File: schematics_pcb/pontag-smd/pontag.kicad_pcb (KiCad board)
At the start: 2 copper layers, 31 parts, among them J1 External 5V, J2 External 12V, J3 RS232 Port, J4 PS/2 Mouse, J5 ISP, J7 Extra, SW1 Reset, U1 LP2985-5.0, U3 ATmega8A-AU, U4 MAX232A, Y1 8.0Mhz

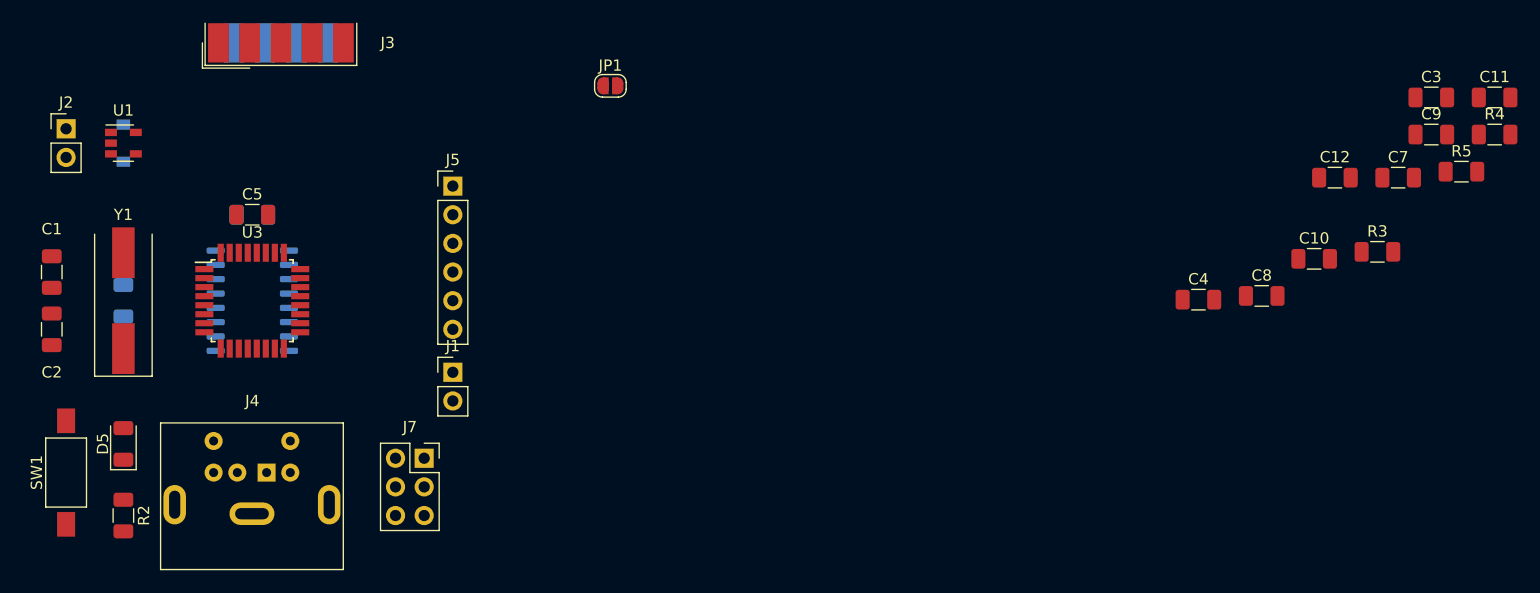
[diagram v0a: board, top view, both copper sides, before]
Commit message: Go on with board routing
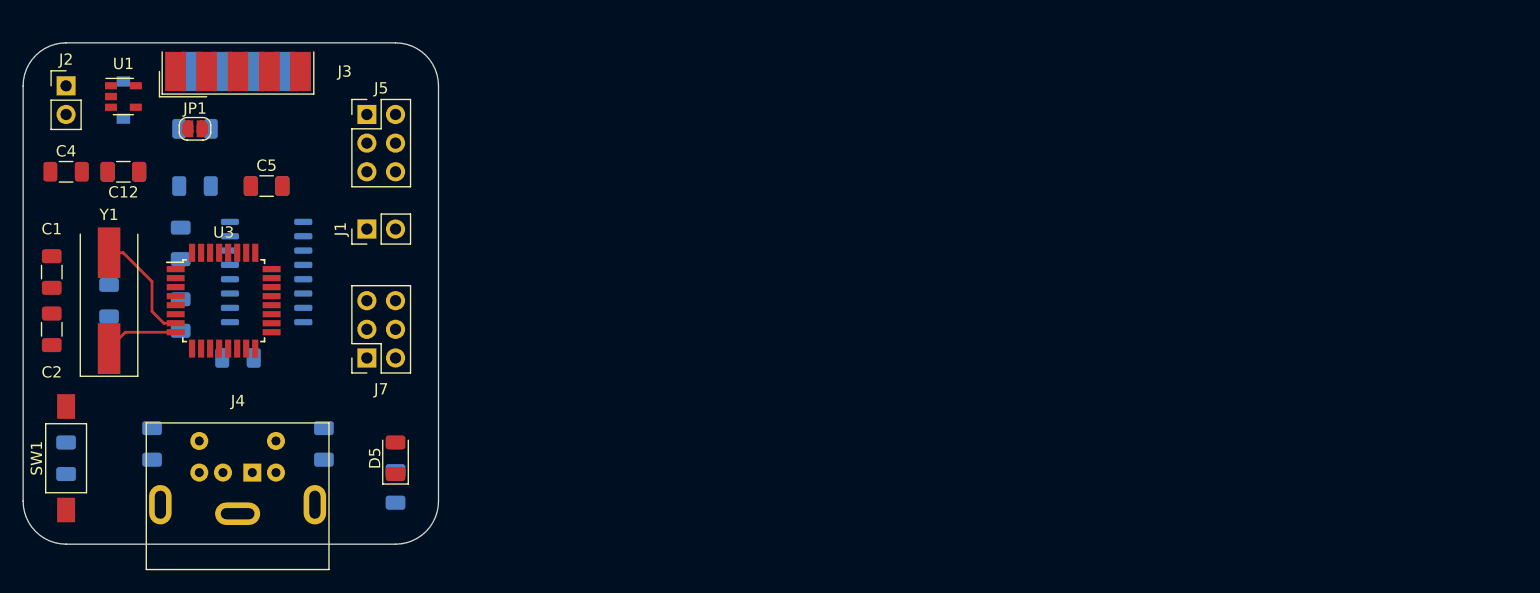
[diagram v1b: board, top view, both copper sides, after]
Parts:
- C10, C11, C3, C7, C8, C9, R2, R3, R4, R5: moved to B.Cu
- J5: value ISP -> AVR-ISP-6; footprint Connector_PinHeader_2.54mm:PinHeader_1x06_P2.54mm_Vertical -> Connector_PinHeader_2.54mm:PinHeader_2x03_P2.54mm_Vertical
- moved R5 126.3 mm to (67.3, 133.3), turned to 270 degrees
- moved C3 116.2 mm to (72.4, 108.0)
- moved C11 115.5 mm to (78.7, 109.2)
- moved C9 111.3 mm to (77.5, 114.3), turned to 90 degrees
- moved R3 110.0 mm to (74.9, 132.1), turned to 90 degrees
- moved C12 107.4 mm to (72.4, 108.0), turned to 180 degrees
- moved R4 107.4 mm to (90.2, 132.1), turned to 270 degrees
- moved C7 106.8 mm to (78.7, 104.1), turned to 180 degrees
- moved C4 101.0 mm to (67.3, 108.0)
- moved C8 95.9 mm to (77.5, 120.7), turned to 90 degrees
- moved C10 95.8 mm to (82.5, 124.5)
- moved JP1 37.0 mm to (78.7, 104.1)
- moved R2 24.3 mm to (96.5, 135.9)
- moved D5 24.2 mm to (96.5, 133.3)
- moved J1 14.8 mm to (94.0, 113.0), turned to 90 degrees
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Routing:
- net /XTAL1: track 0.00 -> 10.0 mm
- net /XTAL2: track 0.00 -> 6.51 mm
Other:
- board outline added: 36.8 x 44.5 mm

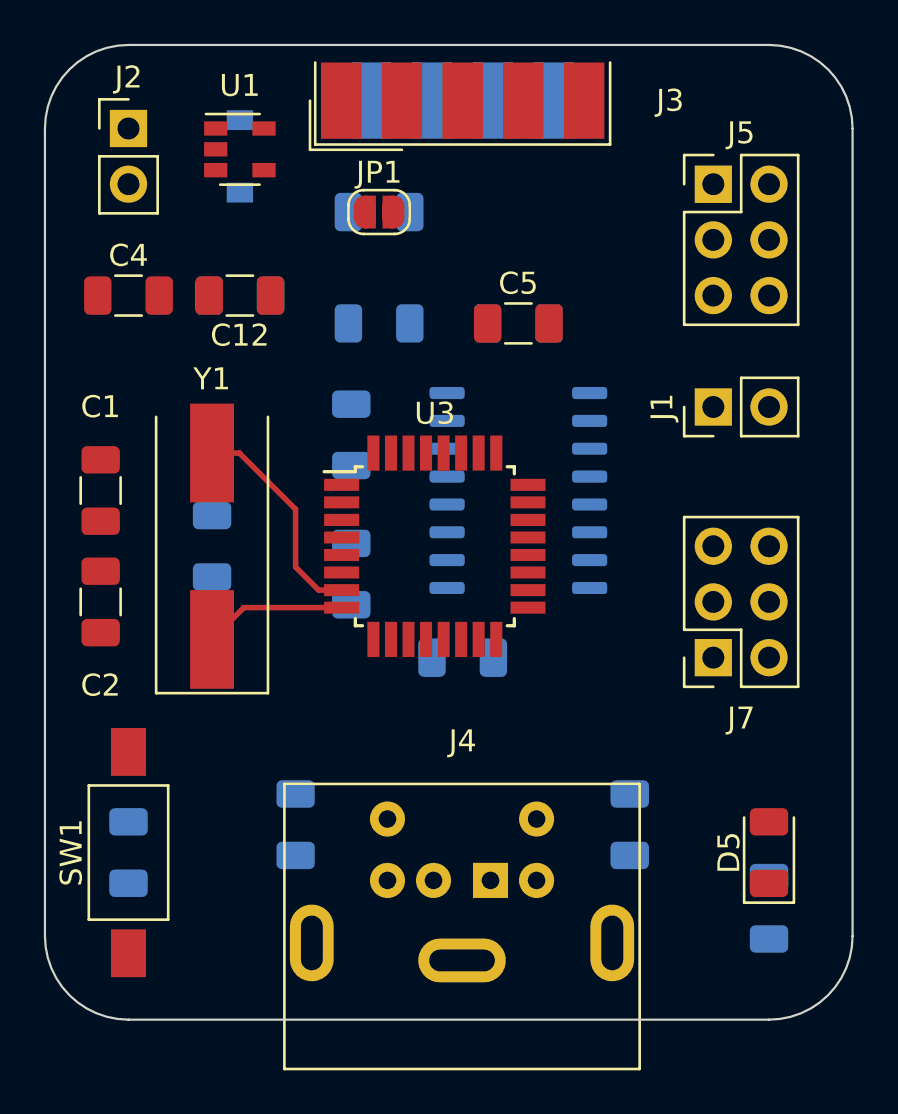
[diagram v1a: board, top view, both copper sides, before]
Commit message: Updates on SMD PCB
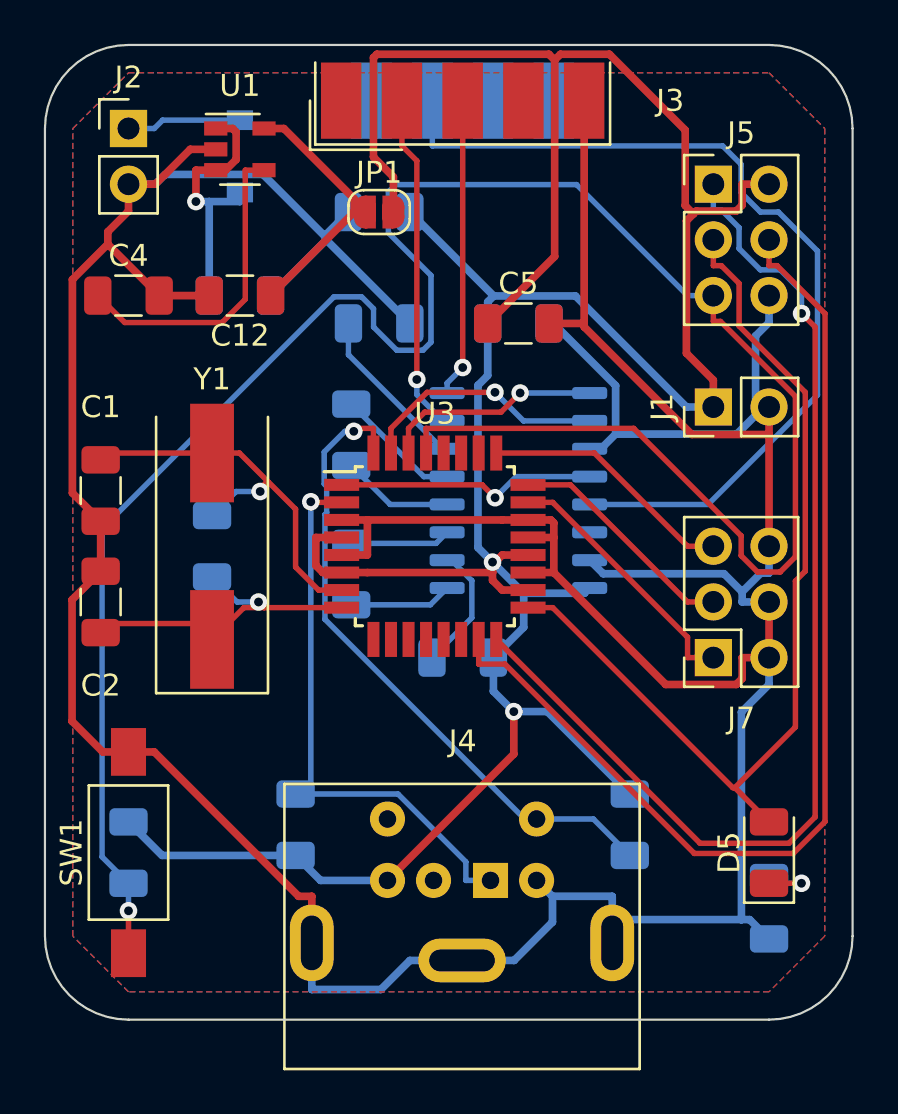
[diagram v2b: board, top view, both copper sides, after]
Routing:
- net GND: track 0.00 -> 210.0 mm
- net VCC: track 0.00 -> 141.2 mm, vias 0 -> 2
- net /RESET: track 0.00 -> 100.7 mm, vias 0 -> 1
- net /MISO: track 0.00 -> 50.4 mm, vias 0 -> 1
- net /MOSI: track 0.00 -> 48.9 mm
- net /SCK: track 0.00 -> 43.3 mm
- net /RS232-RTS: track 0.00 -> 41.4 mm
- net /PS2-CLOCK: track 0.00 -> 29.9 mm, vias 0 -> 1
- net /PS2-DATA: track 0.00 -> 25.8 mm, vias 0 -> 1
- net /RS232-RX: track 0.00 -> 15.6 mm, vias 0 -> 1
- net Net-(C4-Pad1): track 0.00 -> 14.4 mm
- net /RS232-TX: track 0.00 -> 13.6 mm, vias 0 -> 1
- net +12V: track 0.00 -> 12.4 mm, vias 0 -> 1
- net /TTL-CTS: track 0.00 -> 12.0 mm, vias 0 -> 1
- net Net-(J7-Pad1): track 0.00 -> 11.9 mm
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- added copper zone on B.Cu, net GND
- added copper zone on F.Cu, net GND
